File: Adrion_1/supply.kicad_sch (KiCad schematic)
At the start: 17 parts, among them IC2 L6986H, IC3 TPS7A2030PDBVR

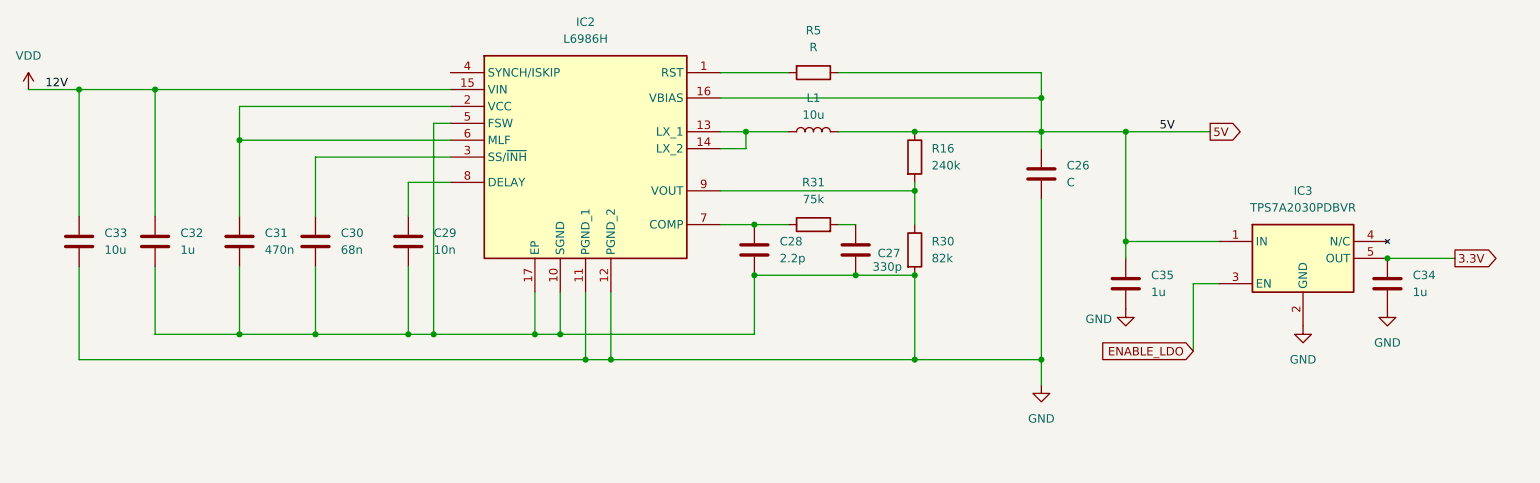
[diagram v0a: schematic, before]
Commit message: Modificaciones
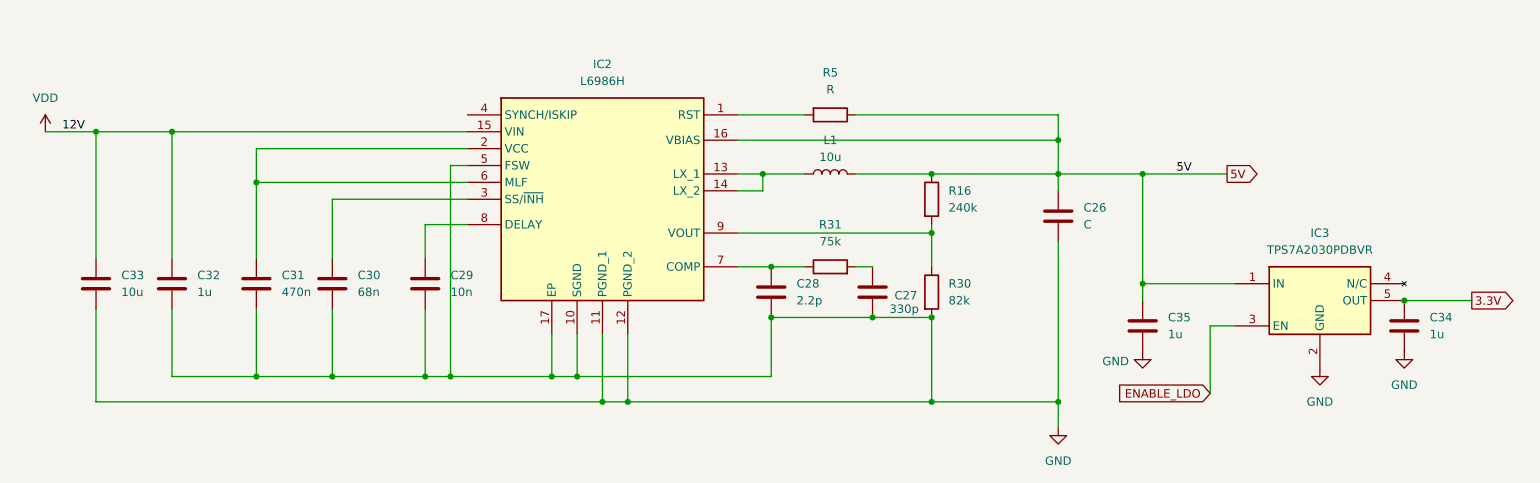
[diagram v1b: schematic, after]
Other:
- moved on the sheet: C26, C27, C28, C29, C30, C31, C32, C33, C34, C35, IC2, IC3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
